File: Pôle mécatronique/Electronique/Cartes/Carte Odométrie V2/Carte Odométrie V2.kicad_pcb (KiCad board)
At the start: 2 copper layers, 72 x 86.2 mm, 14 parts, among them J1 Conn_01x08, J5 Conn_01x07, U1 TCAN332

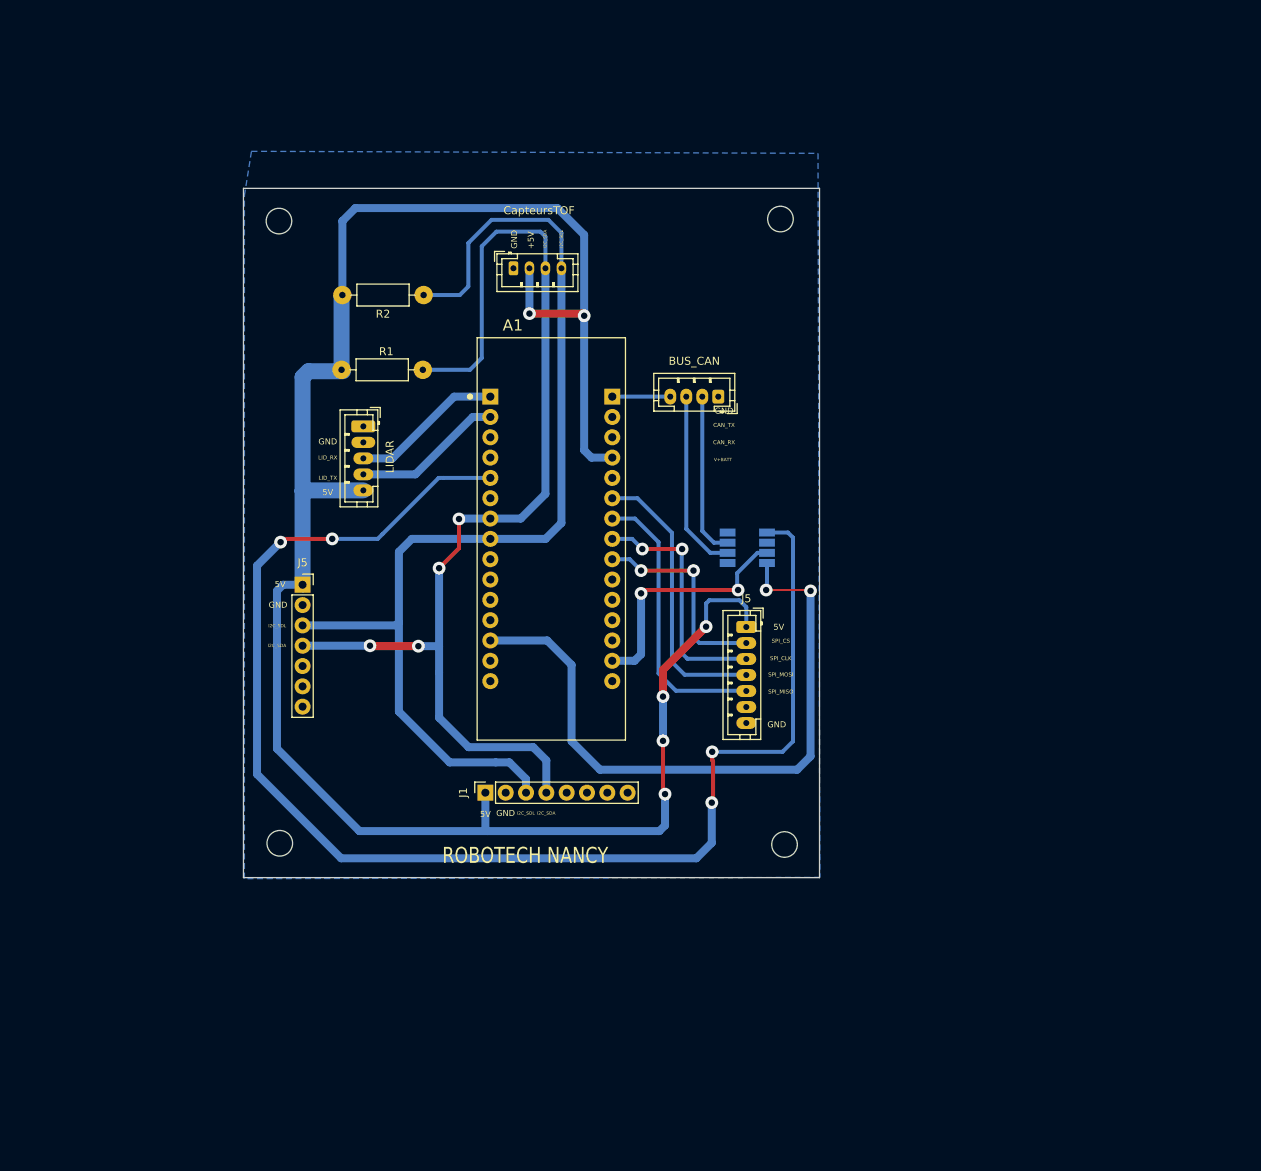
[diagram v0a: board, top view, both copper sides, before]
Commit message: MAJ carte actionneur
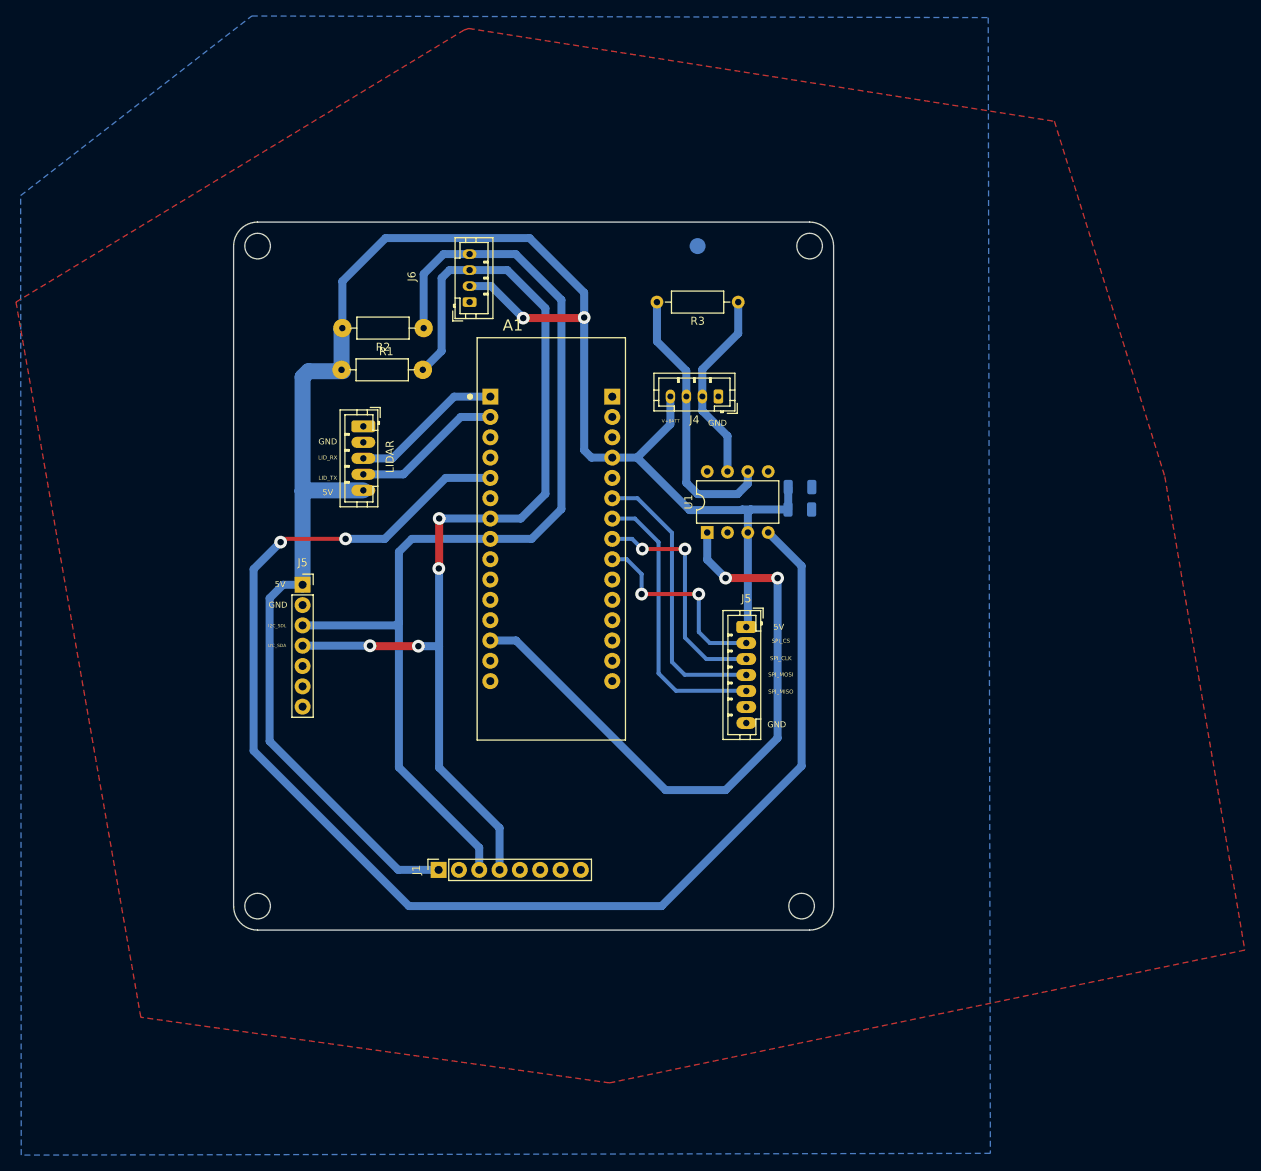
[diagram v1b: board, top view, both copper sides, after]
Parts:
- removed BUS_CAN: Conn_01x04, Connector_JST:JST_PH_B4B-PH-K_1x04_P2.00mm_Vertical
- added C1: C, Capacitor_SMD:C_1206_3216Metric, B.Cu at (199.8, 95.1)
- added C2: C, Capacitor_SMD:C_1206_3216Metric, B.Cu at (199.8, 97.9)
- added J4: Conn_01x04, Connector_JST:JST_PH_B4B-PH-K_1x04_P2.00mm_Vertical, F.Cu at (189.6, 83.8)
- added R3: R, Resistor_THT:R_Axial_DIN0207_L6.3mm_D2.5mm_P10.16mm_Horizontal, F.Cu at (192.1, 72.0)
- added TP1: TestPoint, TestPoint:TestPoint_Pad_D2.0mm, B.Cu at (187.0, 65.0)
- U1: value TCAN332 -> MCP2551-I-P; footprint empreinte:SO-8_S -> Package_DIP:DIP-8_W7.62mm; moved to F.Cu
- moved J1 11.3 mm to (154.6, 143.0)
- moved REF 8.33 mm to (132.0, 147.5)
- moved REF 7.99 mm to (200.0, 147.5)
- moved J6 6.92 mm to (158.5, 72.0), turned to 90 degrees
- moved U1 5.36 mm to (188.2, 100.8), turned to 90 degrees
- moved REF 4.97 mm to (201.0, 65.0)
- moved R2 4.13 mm to (152.8, 75.2)
- moved REF 4.11 mm to (132.0, 65.0)
- renumbered CapteursTOF to J6
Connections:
- A1 pad 4.1: +BATT -> unconnected-(A1-Pad4.1)
- U1 pad 1: CAN_RX -> CAN_TX
- U1 pad 3: +3V3 -> +5V
- U1 pad 4: CAN_TX -> CAN_RX
- U1 pad 8: unconnected-(U1-Pad8) -> GND
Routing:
- net +3V3: track 30.5 -> 0.00 mm, vias 2 -> 0
- net +5V: track 252.6 -> 227.2 mm, vias 6 -> 2
- net CAN_L: track 22.9 -> 34.5 mm
- net I2C_SDA: track 137.8 -> 129.8 mm
- net +BATT: track 7.25 -> 0.00 mm
- net I2C_SCL: track 136.3 -> 132.2 mm
- net CAN_H: track 20.6 -> 24.3 mm
- net CAN_TX: track 82.5 -> 79.5 mm
- net SPI_CLK: track 30.8 -> 29.5 mm
- net SPI_CS: track 26.5 -> 25.3 mm
- net CAN_RX: track 172.9 -> 171.7 mm, vias 4 -> 2
- added copper zone on F.Cu, net GND
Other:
- board size 72 x 86.2 mm -> 75 x 88.5 mm
- board text removed: "+5V"
- board text removed: "CAN_RX"
- board text removed: "CAN_TX"
- board text removed: "ROBOTECH NANCY"
